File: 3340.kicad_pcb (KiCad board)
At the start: 2 copper layers, 50.8 x 106.7 mm, 181 parts, among them J1 Conn_01x16, J10 FM1, J11 Conn_01x16, J12 V/OCT2, J13 PULSE2, J14 SAW2, J15 TRI2, J16 SINE2, J17 SYNC2, J18 Conn_01x16, J19 PWM2, J2 Conn_01x16, J20 FM2, J3 V/OCT1, J4 PULSE1, J5 SAW1, J6 TRI1, J7 SINE1, J8 SYNC1, J9 PWM1, Q1 2N3904, Q2 2N3906, Q3 2N3904, Q4 2N3906, Q5 2N3904, Q6 2N3904, SW2 DPDT_OOO, U1 TL072, U2 TL074, U3 CEM3340, U4 TL072, U5 CEM3340, U6 TL074

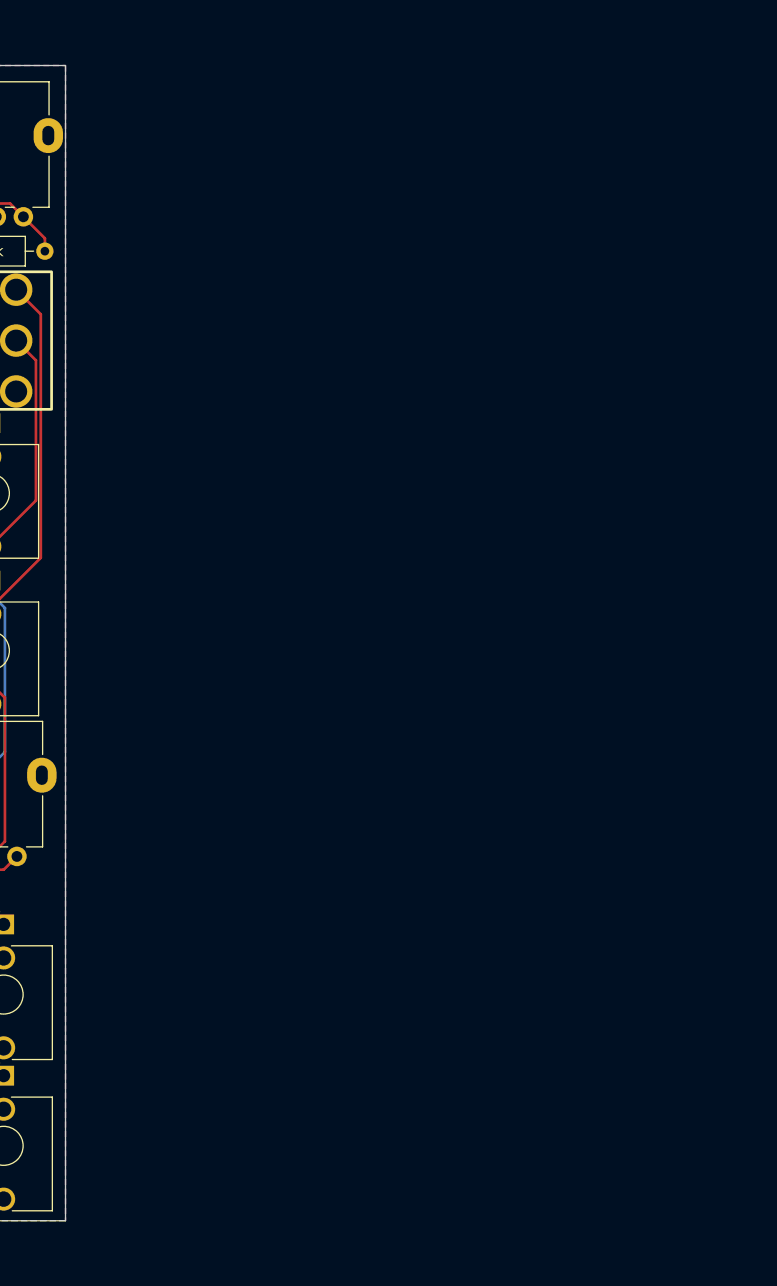
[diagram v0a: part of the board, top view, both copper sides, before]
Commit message: Fix power routing
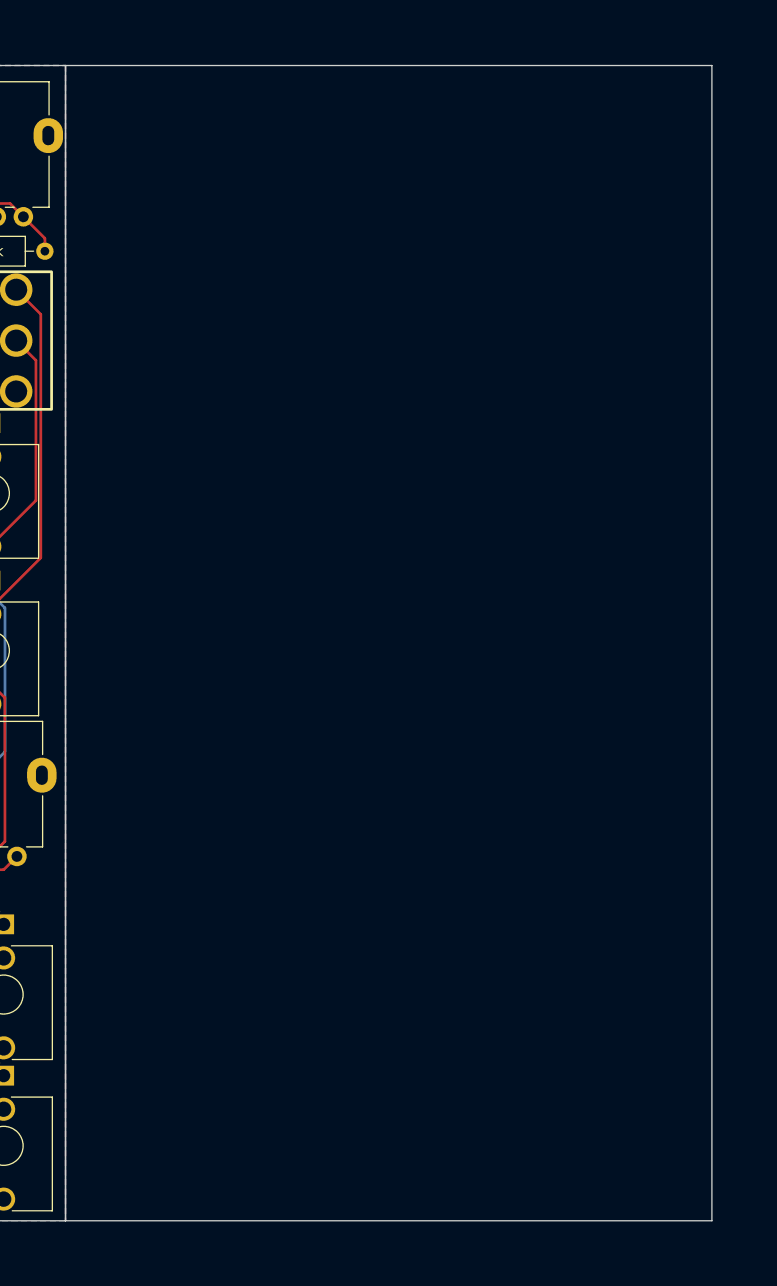
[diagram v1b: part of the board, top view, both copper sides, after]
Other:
- board size 50.8 x 106.7 mm -> 110.5 x 106.7 mm
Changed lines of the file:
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@@
   (gr_rect (start -110.49 31.75) (end -99.06 138.43) (layer "F.SilkS") (width 0.15) (fill none))
   (gr_rect (start 12.7 12.7) (end 63.5 119.38) (layer "Edge.Cuts") (width 0.1) (fill none))
+  (gr_rect (start 63.5 12.7) (end 123.19 119.38) (layer "Edge.Cuts") (width 0.1) (fill none))
   (segment (start 49.28601 50.8) (end 46.99 50.8) (width 0.25) (layer "B.Cu") (net 1))
   (segment (start 41.99 43.825) (end 45.155 46.99) (width 0.25) (layer "B.Cu") (net 1))
